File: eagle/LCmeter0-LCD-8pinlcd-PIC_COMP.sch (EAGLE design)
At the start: 34 parts, among them IC1 PIC16F876A-X/SP-COMP-B-A, J1 HD44780-4BIT-8PIN, J2 PIC-UART, J3 PIC-ICSPICSP, K2 DS2Y, Q1 20MHz, T1 BC547CBE-A, X1 FREQ, X2 L/C

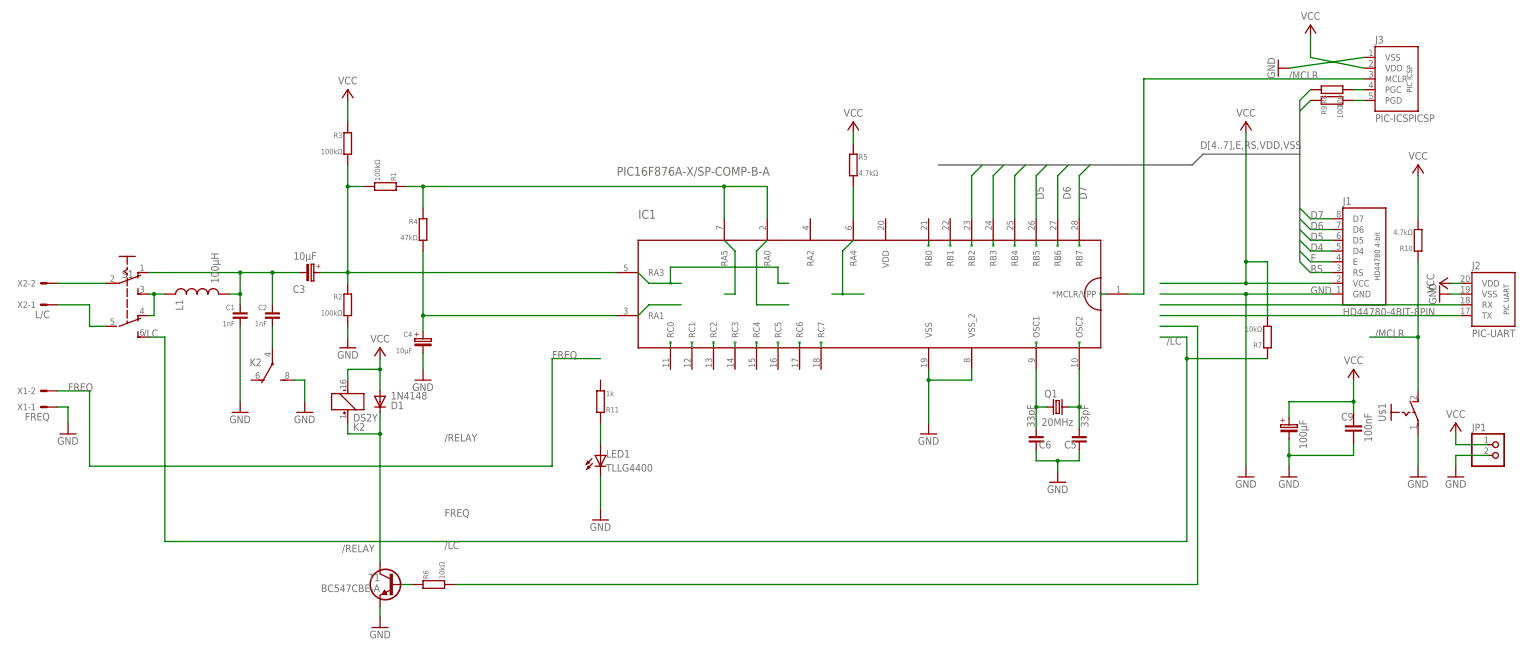
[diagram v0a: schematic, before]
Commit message: ...
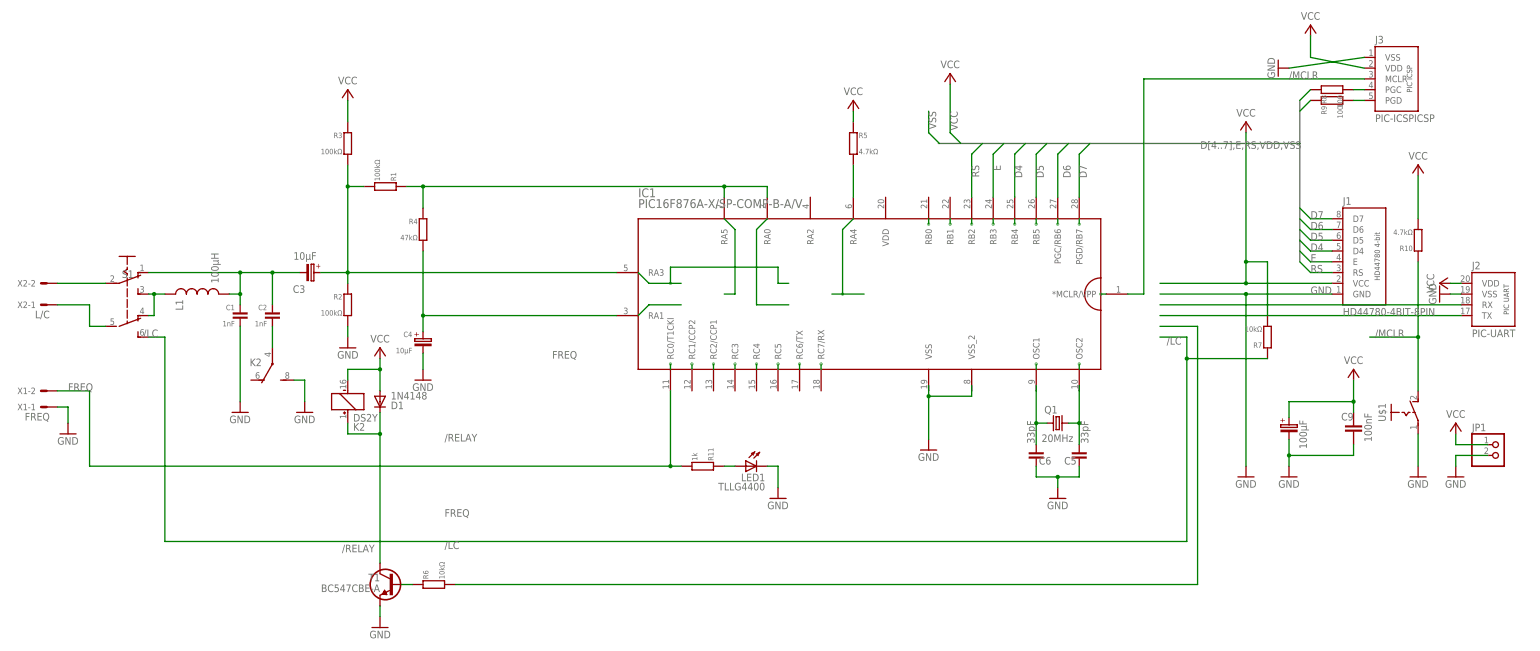
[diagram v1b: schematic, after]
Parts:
- IC1: value PIC16F876A-X/SP-COMP-B-A -> PIC16F876A-X/SP-COMP-B-A/V; device mcu:PIC16F876A-X/SP-COMP-B-A -> mcu:PIC16F876A-X/SP-COMP-B-A/V
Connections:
- net D6: now also IC1.PGC/RB6; no longer IC1.RB6
- net D7: now also IC1.PGD/RB7; no longer IC1.RB7
- net FREQ: now also IC1.RC0/T1CKI, R11.2
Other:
- moved on the sheet: C5, C6, LED1, Q1, R11, R5
